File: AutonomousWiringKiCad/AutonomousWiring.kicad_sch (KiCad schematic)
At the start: 31 parts

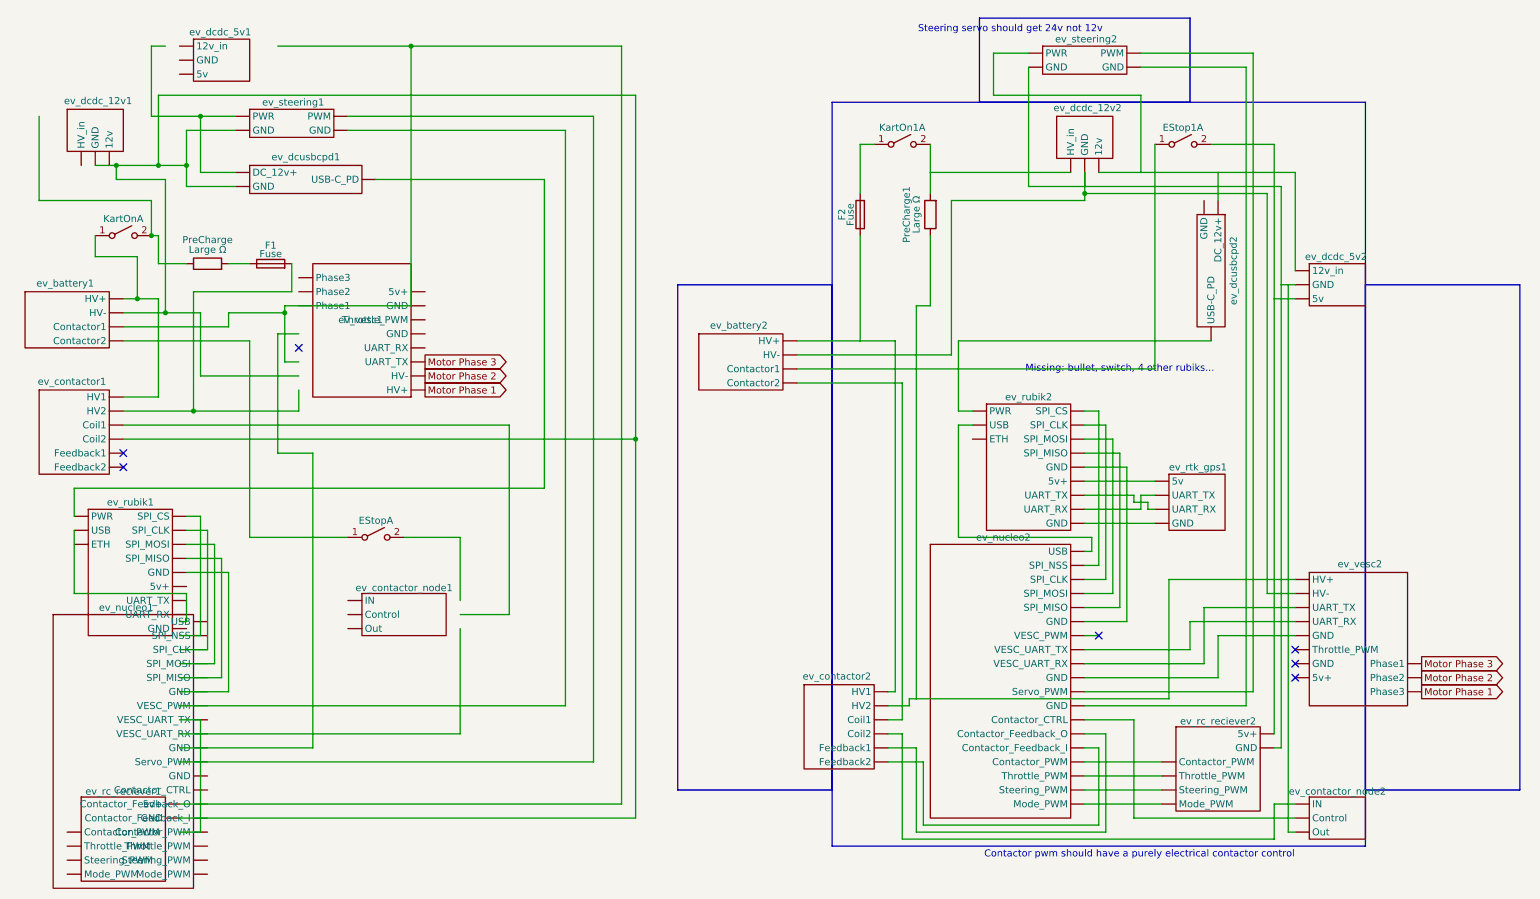
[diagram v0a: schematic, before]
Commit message: Removing old draft
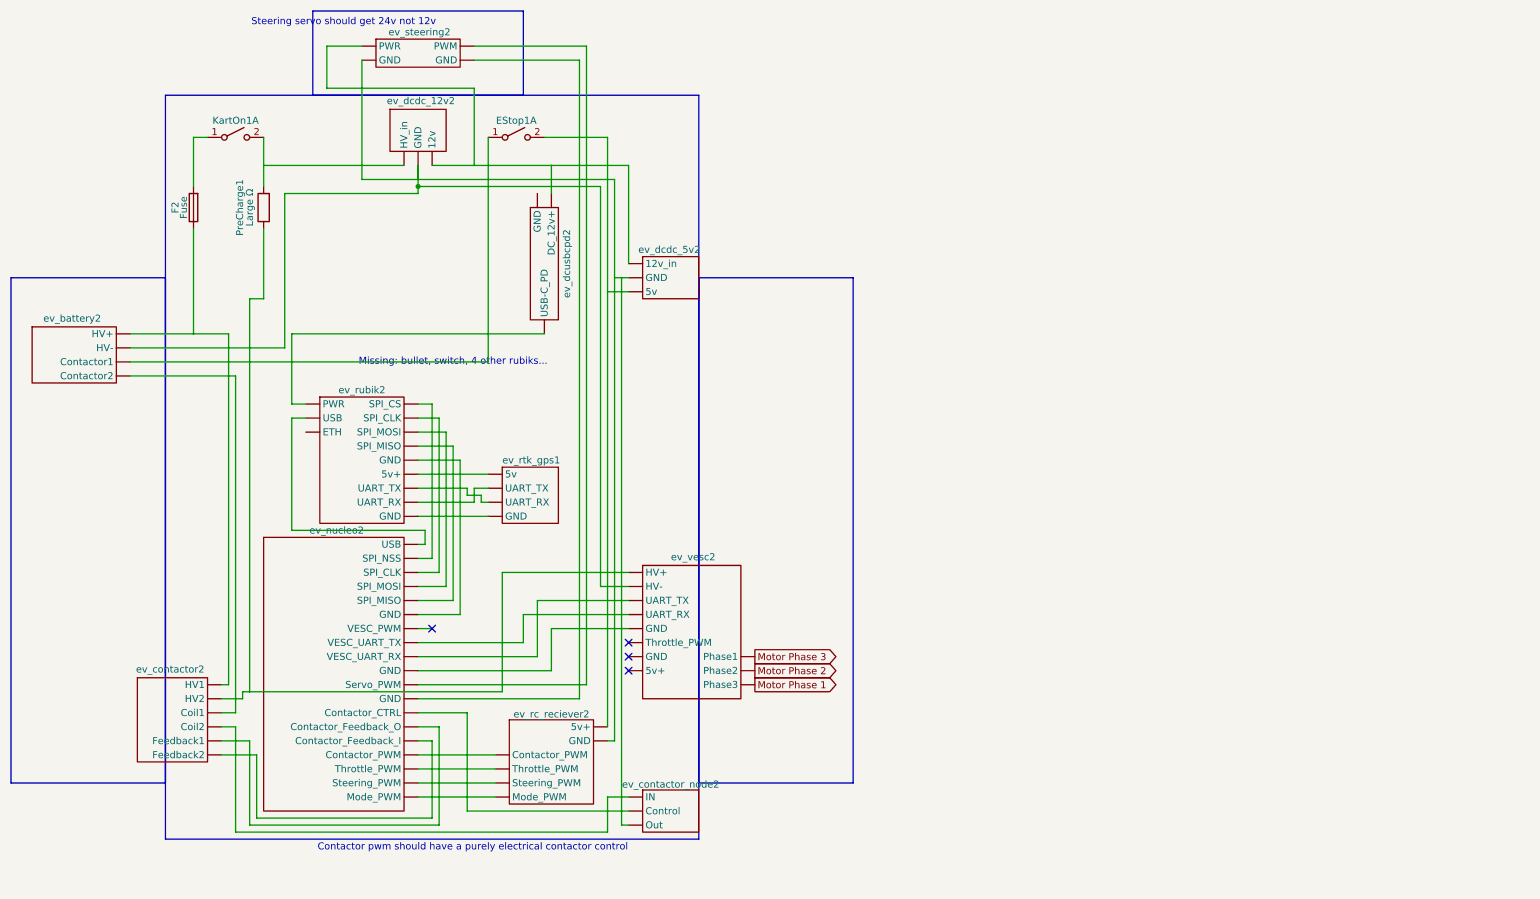
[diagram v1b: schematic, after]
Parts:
- removed EStop, KartOn: SW_DPST_x2, symbol Switch:SW_DPST_x2
- removed F1: Fuse, symbol Device:Fuse
- removed PreCharge: Large Ω, symbol Device:R
- removed ev_battery1: ~, symbol ev_kart:ev_battery
- removed ev_contactor1: ~, symbol ev_kart:ev_contactor
- removed ev_contactor_node1: ~, symbol ev_kart:ev_contactor_node
- removed ev_dcdc_12v1: ~, symbol ev_kart:ev_dcdc_12v
- removed ev_dcdc_5v1: ~, symbol ev_kart:ev_dcdc_5v
- removed ev_dcusbcpd1: ~, symbol ev_kart:ev_dcusbcpd
- removed ev_nucleo1: ~, symbol ev_kart:ev_nucleo
- removed ev_rc_reciever1: ~, symbol ev_kart:ev_rc_reciever
- removed ev_rubik1: ~, symbol ev_kart:ev_rubik
- removed ev_steering1: ~, symbol ev_kart:ev_steering
- removed ev_vesc1: ~, symbol ev_kart:ev_vesc
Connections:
- net at ev_nucleo2. (Mode_PWM): now also ev_vesc2. (Phase3)
- net at ev_contactor_node2. (Out): now also ev_contactor2. (Feedback2); no longer ev_nucleo2. (Mode_PWM)
- net at ev_steering2. (GND): now also ev_dcdc_12v2. (12v), ev_dcdc_5v2. (5v), ev_dcusbcpd2. (USB-C_PD); no longer ev_nucleo2. (Mode_PWM)
- net at ev_contactor2. (Feedback2): now also PreCharge1.1, ev_vesc2. (Phase3); no longer ev_nucleo2. (Mode_PWM)
- net at ev_rc_reciever2. (GND): now also EStop1.2 (B), ev_dcdc_5v2. (5v); no longer ev_nucleo2. (Mode_PWM)
- net at ev_rubik2. (GND): no longer ev_nucleo2. (Mode_PWM)
- net at ev_battery2. (Contactor2): now also EStop1.1 (A); no longer ev_contactor2. (Feedback2)
- net at ev_dcusbcpd2. (USB-C_PD): now also ev_rubik2. (GND)
- new net: ev_contactor_node2. (Out), ev_nucleo2. (Mode_PWM)
- new net: ev_nucleo2. (Mode_PWM), ev_steering2. (GND) (x2)
- new net: ev_contactor2. (Feedback2), ev_nucleo2. (Mode_PWM) (x2)
- new net: ev_nucleo2. (Mode_PWM), ev_rc_reciever2. (GND) (x4)
- new net: ev_nucleo2. (Mode_PWM), ev_rubik2. (GND) (x6)
- new net: ev_nucleo2. (Mode_PWM), ev_vesc2. (Phase3) (x2)
- new net: F2.1, ev_battery2. (Contactor2), ev_contactor2. (Feedback2)
- new net: ev_battery2. (Contactor2), ev_contactor_node2. (Out), ev_dcdc_12v2. (12v), ev_dcdc_5v2. (5v), ev_rc_reciever2. (GND), ev_steering2. (GND), ev_vesc2. (Phase3)
- new net: ev_battery2. (Contactor2), ev_contactor2. (Feedback2)
- new net: ev_rtk_gps1. (GND), ev_rubik2. (GND) (x3)
- now unconnected: ev_rubik2. (GND), ev_rubik2. (GND), ev_rubik2. (GND), ev_rubik2. (GND), ev_rubik2. (GND), ev_rubik2. (GND), ev_rubik2. (GND), ev_rubik2. (GND), ev_rubik2. (GND)
- no-connect marks 7 -> 4
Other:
- moved on the sheet: EStop1A, F2, KartOn1A, PreCharge1, ev_battery2, ev_contactor2, ev_contactor_node2, ev_dcdc_12v2, ev_dcdc_5v2, ev_dcusbcpd2, ev_nucleo2, ev_rc_reciever2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
